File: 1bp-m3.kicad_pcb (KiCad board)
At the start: 2 copper layers, 27.5 x 24.8 mm, 34 parts, among them J1 TCS7913-43, P13 TP_50, P7 TP_50, P8 TP_50, P9 TP_50, U1 TL972IDR

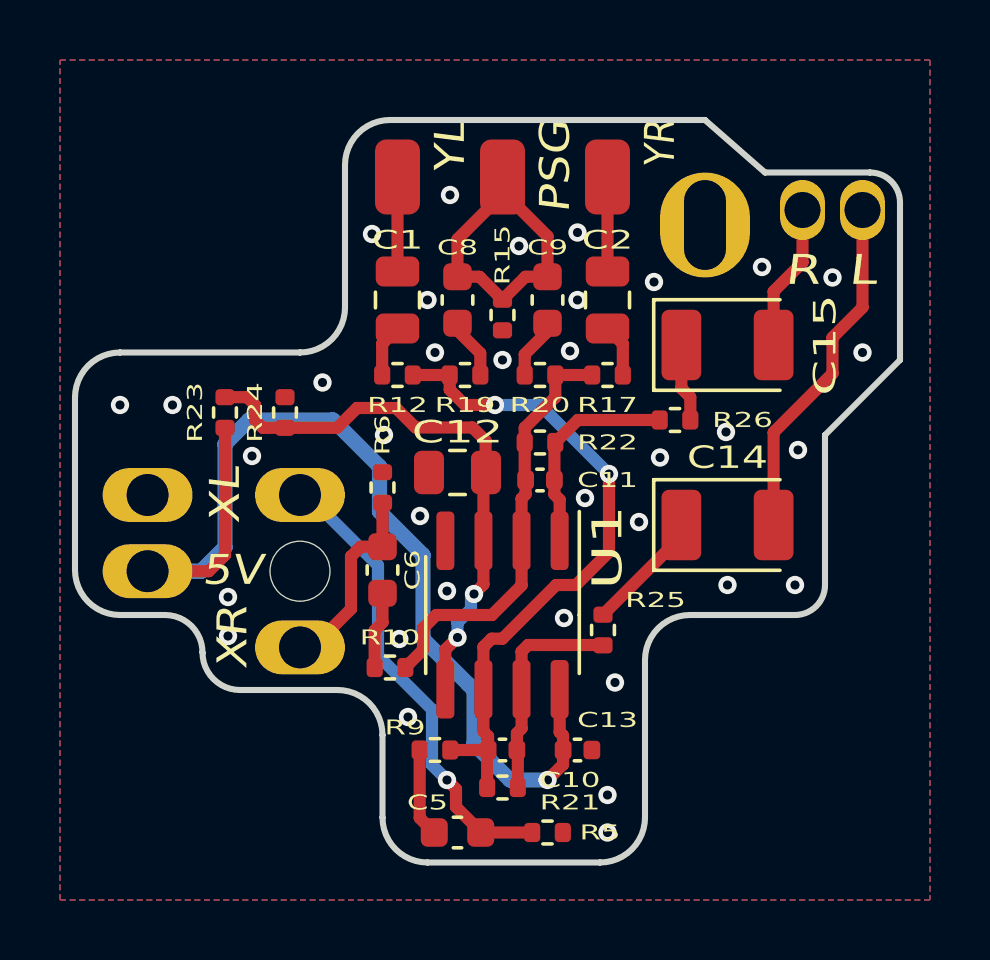
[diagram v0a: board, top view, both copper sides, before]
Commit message: export gerbers
first fab run
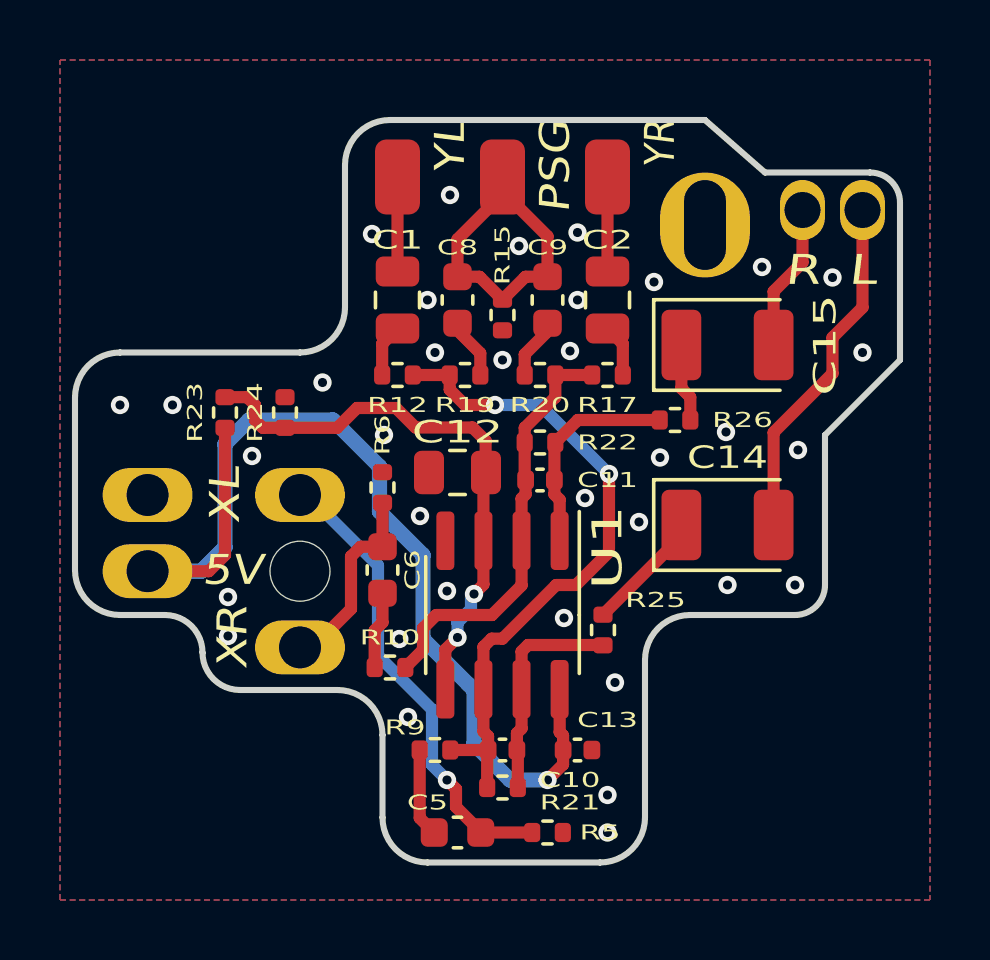
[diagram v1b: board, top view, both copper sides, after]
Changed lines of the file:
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@@
     (solder_mask_min_width 0.25)
     (pcbplotparams
-      (layerselection 0x00012fc_ffffffff)
+      (layerselection 0x00010f8_ffffffff)
       (disableapertmacros false)
       (usegerberextensions false)
-      (usegerberattributes false)
+      (usegerberattributes true)
       (usegerberadvancedattributes false)
       (creategerberjobfile true)
       (svguseinch false)
       (svgprecision 6)
-      (excludeedgelayer false)
-      (plotframeref true)
+      (excludeedgelayer true)
+      (plotframeref false)
       (viasonmask false)
       (mode 1)
@@
   )
   (footprint "Resistor_SMD:R_0402_1005Metric" (layer "F.Cu")
-    (at 129.750007 84.500009 -90)
+    (at 129.75 84.5 -90)
     (descr "Resistor SMD 0402 (1005 Metric), square (rectangular) end terminal, IPC_7351 nominal, (Body size source: IPC-SM-782 page 72, https://www.pcb-3d.com/wordpress/wp-content/uploads/ipc-sm-782a_amendment_1_and_2.pdf), generated with kicad-footprint-generator")
     (tags "resistor")
@@
   )
   (footprint "Resistor_SMD:R_0402_1005Metric" (layer "F.Cu")
-    (at 125.74999 90.25001 90)
+    (at 125.75 90.25 90)
     (descr "Resistor SMD 0402 (1005 Metric), square (rectangular) end terminal, IPC_7351 nominal, (Body size source: IPC-SM-782 page 72, https://www.pcb-3d.com/wordpress/wp-content/uploads/ipc-sm-782a_amendment_1_and_2.pdf), generated with kicad-footprint-generator")
     (tags "resistor")
@@
   )
   (footprint "Capacitor_SMD:C_0603_1608Metric" (layer "F.Cu")
-    (at 128.25001 84.00001 -90)
+    (at 128.25 84 -90)
     (descr "Capacitor SMD 0603 (1608 Metric), square (rectangular) end terminal, IPC_7351 nominal, (Body size source: IPC-SM-782 page 76, https://www.pcb-3d.com/wordpress/wp-content/uploads/ipc-sm-782a_amendment_1_and_2.pdf), generated with kicad-footprint-generator")
     (tags "capacitor")
@@
   )
   (footprint "Capacitor_SMD:C_0402_1005Metric" (layer "F.Cu")
-    (at 132.250002 99.000005)
+    (at 132.25 99)
     (descr "Capacitor SMD 0402 (1005 Metric), square (rectangular) end terminal, IPC_7351 nominal, (Body size source: IPC-SM-782 page 76, https://www.pcb-3d.com/wordpress/wp-content/uploads/ipc-sm-782a_amendment_1_and_2.pdf), generated with kicad-footprint-generator")
     (tags "capacitor")
@@
   )
   (footprint "Package_SO:SOIC-8_3.9x4.9mm_P1.27mm" (layer "F.Cu")
-    (at 129.750007 94.499989 -90)
+    (at 129.75 94.5 -90)
     (descr "SOIC, 8 Pin (JEDEC MS-012AA, https://www.analog.com/media/en/package-pcb-resources/package/pkg_pdf/soic_narrow-r/r_8.pdf), generated with kicad-footprint-generator ipc_gullwing_generator.py")
     (tags "SOIC SO")
@@
   )
   (footprint "Capacitor_SMD:C_0805_2012Metric" (layer "F.Cu")
-    (at 128.25001 89.750011)
+    (at 128.25 89.75)
     (descr "Capacitor SMD 0805 (2012 Metric), square (rectangular) end terminal, IPC_7351 nominal, (Body size source: IPC-SM-782 page 76, https://www.pcb-3d.com/wordpress/wp-content/uploads/ipc-sm-782a_amendment_1_and_2.pdf, https://docs.google.com/spreadsheets/d/1BsfQQcO9C6DZCsRaXUlFlo91Tg2WpOkGARC1WS5S8t0/edit?usp=sharing), generated with kicad-footprint-generator")
     (tags "capacitor")
@@
   )
   (footprint "Capacitor_Tantalum_SMD:CP_EIA-3528-21_Kemet-B" (layer "F.Cu")
-    (at 137.249992 85.500007)
+    (at 137.25 85.5)
     (descr "Tantalum Capacitor SMD Kemet-B (3528-21 Metric), IPC_7351 nominal, (Body size from: http://www.kemet.com/Lists/ProductCatalog/Attachments/253/KEM_TC101_STD.pdf), generated with kicad-footprint-generator")
     (tags "capacitor tantalum")
@@
   (segment (start 127.4 97.65) (end 125.6 95.85) (width 0.4064) (layer "B.Cu") (net 6))
   (segment (start 127.4 99.5) (end 127.4 97.65) (width 0.4064) (layer "B.Cu") (net 6))
-  (segment (start 123.25 90.5) (end 123 90.5) (width 0.4064) (layer "B.Cu") (net 6))
   (segment (start 125.6 92.85) (end 123.25 90.5) (width 0.4064) (layer "B.Cu") (net 6))
   (segment (start 125.6 95.85) (end 125.6 92.85) (width 0.4064) (layer "B.Cu") (net 6))
@@
   (segment (start 129.01 86.5) (end 129.01 85.7725) (width 0.4064) (layer "F.Cu") (net 17))
   (segment (start 129.01 85.7725) (end 128.25001 85.01251) (width 0.4064) (layer "F.Cu") (net 17))
-  (segment (start 128.25001 85.01251) (end 128.25001 84.77501) (width 0.4064) (layer "F.Cu") (net 17))
   (segment (start 131.25 83.225) (end 130.515 83.225) (width 0.4064) (layer "F.Cu") (net 18))
   (segment (start 128.25 83.225) (end 128.25 81.975) (width 0.4064) (layer "F.Cu") (net 18))
